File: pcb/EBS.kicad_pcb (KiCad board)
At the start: 2 copper layers, 44.4 x 27.4 mm, 21 parts, among them Q1 BC547, Q2 BC557

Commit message: Change resistor unit
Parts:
- R1, R2: value 10M -> 10Meg
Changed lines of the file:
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@@
         (effects (font (size 1 1) (thickness 0.15)))
     )
-    (fp_text value "10M" (at 0 -1.143 90) (layer "F.Fab")
+    (fp_text value "10Meg" (at -1.016 -1.143 90) (layer "F.Fab")
         (effects (font (size 1 1) (thickness 0.15)))
     )
@@
         (effects (font (size 1 1) (thickness 0.15)))
     )
-    (fp_text value "10M" (at 10.16 1.143 90) (layer "F.Fab")
+    (fp_text value "10Meg" (at 11.176 1.143 90) (layer "F.Fab")
         (effects (font (size 1 1) (thickness 0.15)))
     )
@@
     (pts (xy 147.828 75.819) (xy 147.828 70.485))
     (height 10.922)
-    (gr_text "5.33" (at 157.6 73.152 90) (layer "Dwgs.User")
+    (gr_text "5,33" (at 157.6 73.152 90) (layer "Dwgs.User")
       (effects (font (size 1 1) (thickness 0.15)))
     )
@@
     (pts (xy 147.828 75.565) (xy 106.68 75.565))
     (height 17.145)
-    (gr_text "41.15" (at 127.254 57.27) (layer "Dwgs.User")
+    (gr_text "41,15" (at 127.254 57.27) (layer "Dwgs.User")
       (effects (font (size 1 1) (thickness 0.15)))
     )
@@
     (pts (xy 110.49 74.93) (xy 110.49 70.485))
     (height -11.43)
-    (gr_text "4.45" (at 97.91 72.7075 90) (layer "Dwgs.User")
+    (gr_text "4,45" (at 97.91 72.7075 90) (layer "Dwgs.User")
       (effects (font (size 1 1) (thickness 0.15)))
     )
@@
     (pts (xy 110.49 81.412) (xy 110.49 87.889))
     (height 11.43)
-    (gr_text "6.48" (at 97.91 84.6505 90) (layer "Dwgs.User")
+    (gr_text "6,48" (at 97.91 84.6505 90) (layer "Dwgs.User")
       (effects (font (size 1 1) (thickness 0.15)))
     )
@@
     (pts (xy 106.68 97.917) (xy 106.68 70.485))
     (height -12.7)
-    (gr_text "27.43" (at 92.83 84.201 90) (layer "Dwgs.User")
+    (gr_text "27,43" (at 92.83 84.201 90) (layer "Dwgs.User")
       (effects (font (size 1 1) (thickness 0.15)))
     )
@@
     (pts (xy 110.49 74.93) (xy 110.49 81.412))
     (height 11.43)
-    (gr_text "6.48" (at 97.91 78.171 90) (layer "Dwgs.User")
+    (gr_text "6,48" (at 97.91 78.171 90) (layer "Dwgs.User")
       (effects (font (size 1 1) (thickness 0.15)))
     )
@@
     (pts (xy 110.49 87.889) (xy 110.49 94.361))
     (height 11.43)
-    (gr_text "6.47" (at 97.91 91.125 90) (layer "Dwgs.User")
+    (gr_text "6,47" (at 97.91 91.125 90) (layer "Dwgs.User")
       (effects (font (size 1 1) (thickness 0.15)))
     )
@@
     (pts (xy 110.49 74.93) (xy 106.68 74.93))
     (height 11.43)
-    (gr_text "3.81" (at 108.585 62.35) (layer "Dwgs.User")
+    (gr_text "3,81" (at 108.585 62.35) (layer "Dwgs.User")
       (effects (font (size 1 1) (thickness 0.15)))
     )
@@
     (pts (xy 106.68 70.485) (xy 151.13 70.485))
     (height 36.195)
-    (gr_text "44.45" (at 128.905 105.53) (layer "Dwgs.User")
+    (gr_text "44,45" (at 128.905 105.53) (layer "Dwgs.User")
       (effects (font (size 1 1) (thickness 0.15)))
     )

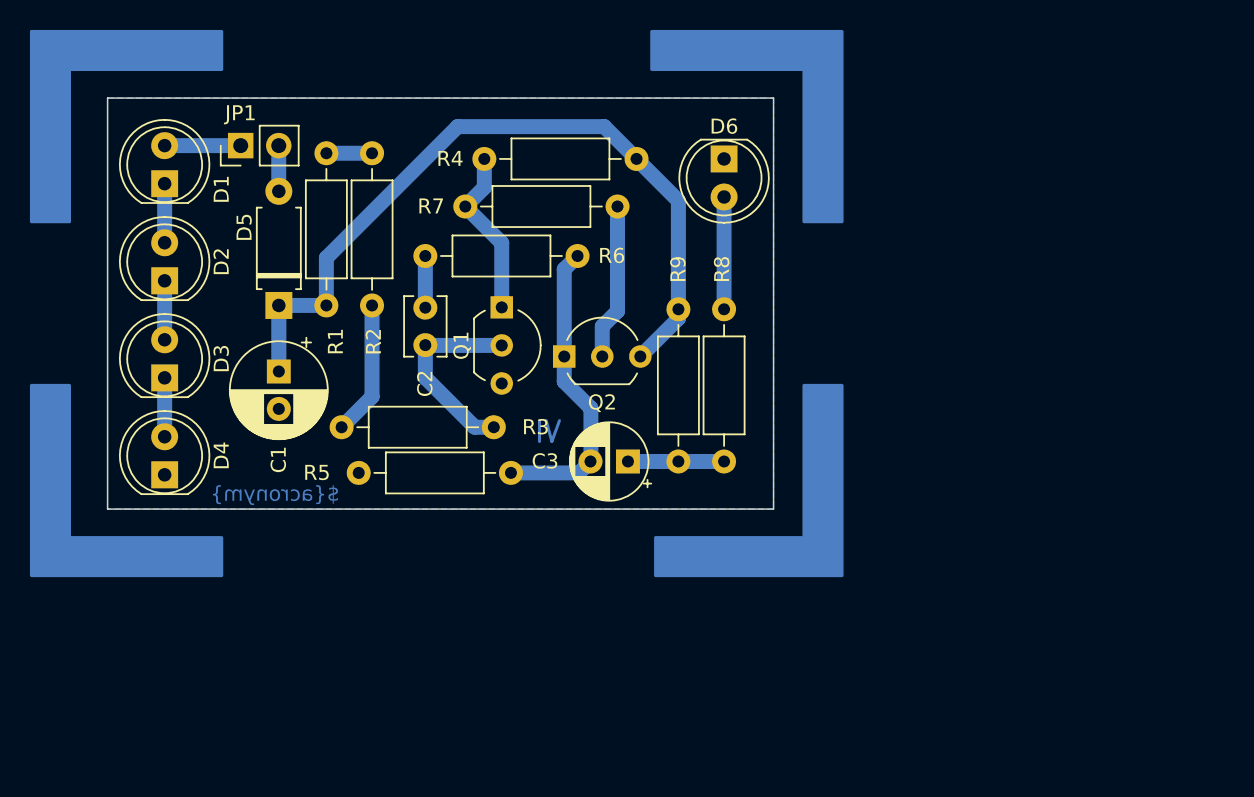
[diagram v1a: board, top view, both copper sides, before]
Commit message: Change 3d models
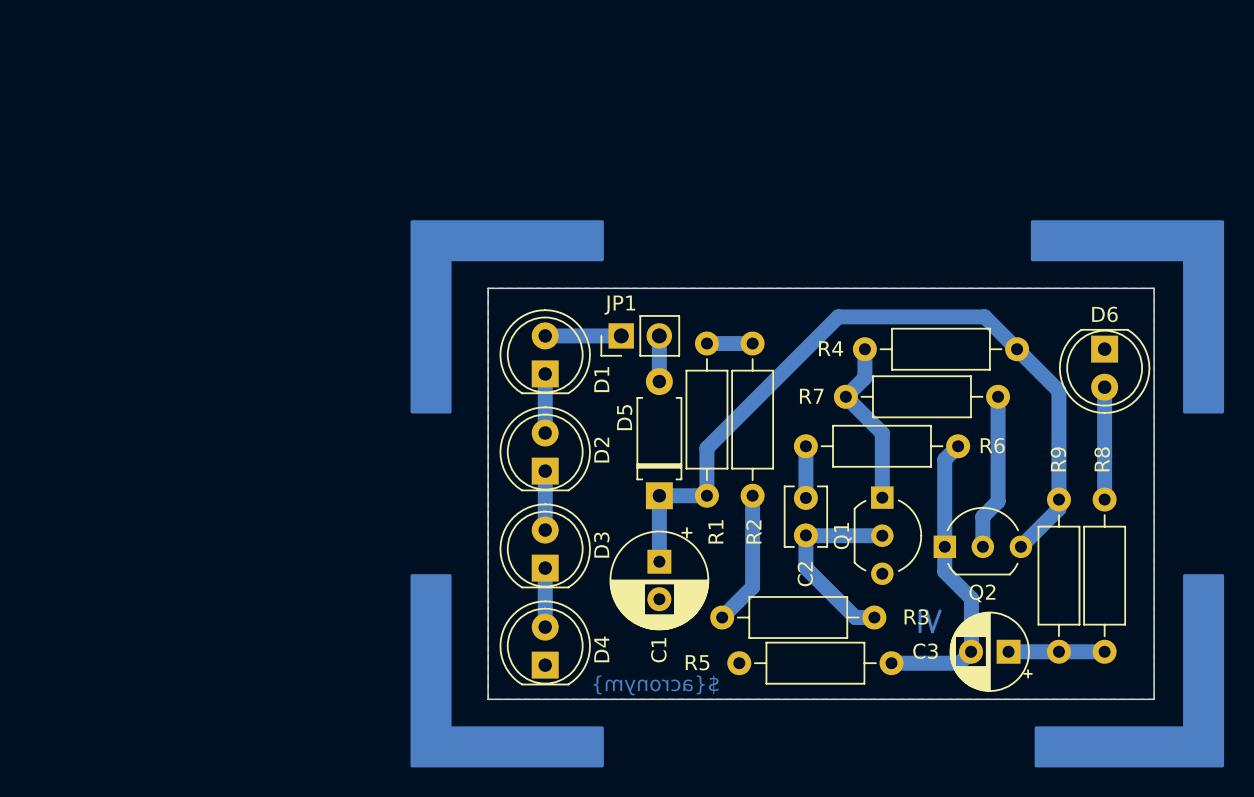
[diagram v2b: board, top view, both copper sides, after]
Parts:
- moved D4 28.4 mm to (135.9, 108.3)
- moved JP1 28.4 mm to (141.0, 86.4)
- moved Q2 28.4 mm to (162.6, 100.4)
- moved R1 28.4 mm to (146.7, 97.0)
- moved R9 28.4 mm to (170.2, 97.3)
- moved R2 28.4 mm to (149.7, 86.9)
- moved R4 28.4 mm to (167.4, 87.2)
- moved R8 28.4 mm to (173.2, 107.4)
- moved C1 28.4 mm to (143.5, 101.4)
- moved C2 28.4 mm to (153.3, 99.7)
- moved D1 28.4 mm to (135.9, 88.9)
- moved D2 28.4 mm to (135.9, 95.4)
- moved D5 28.4 mm to (143.5, 97.0)
- moved R3 28.4 mm to (147.7, 105.2)
- moved R6 28.4 mm to (153.3, 93.7)
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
